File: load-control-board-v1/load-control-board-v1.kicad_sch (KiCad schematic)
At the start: 10 parts, among them Q1 BSC026N08NS5, U1 LM741

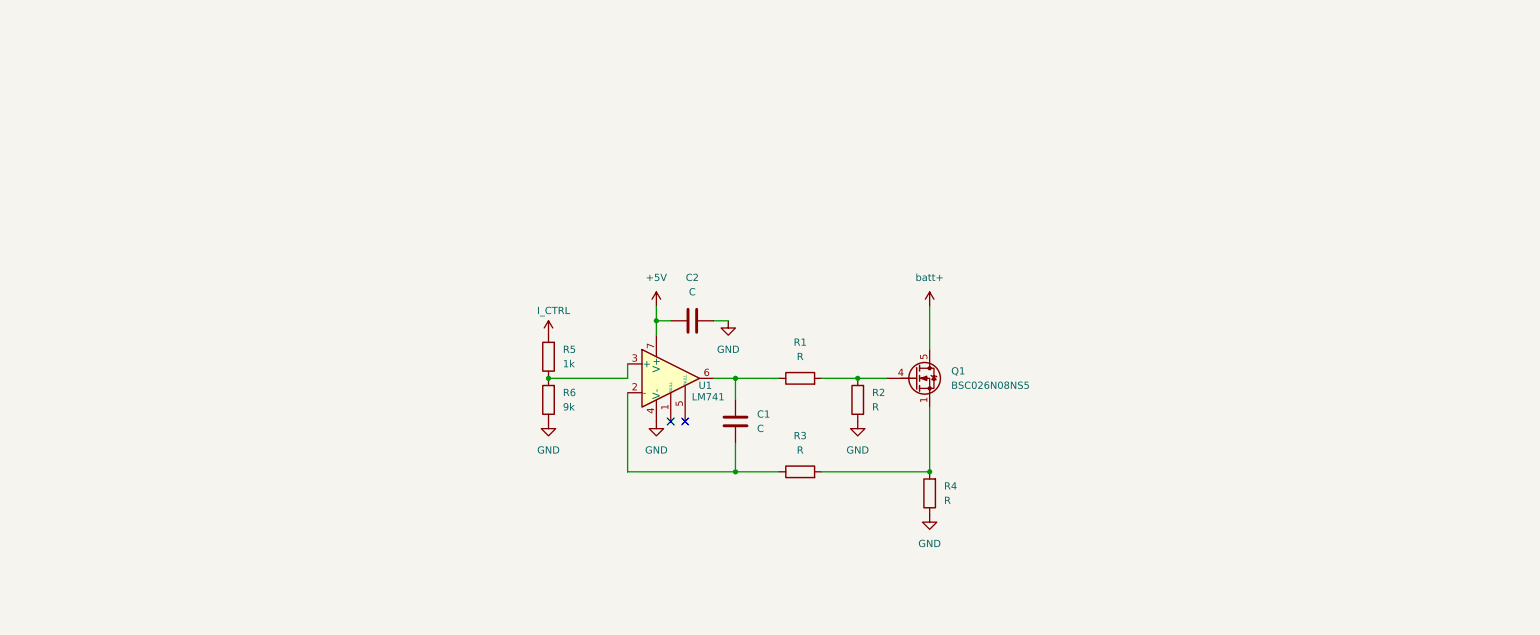
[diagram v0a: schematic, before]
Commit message: communicate 1
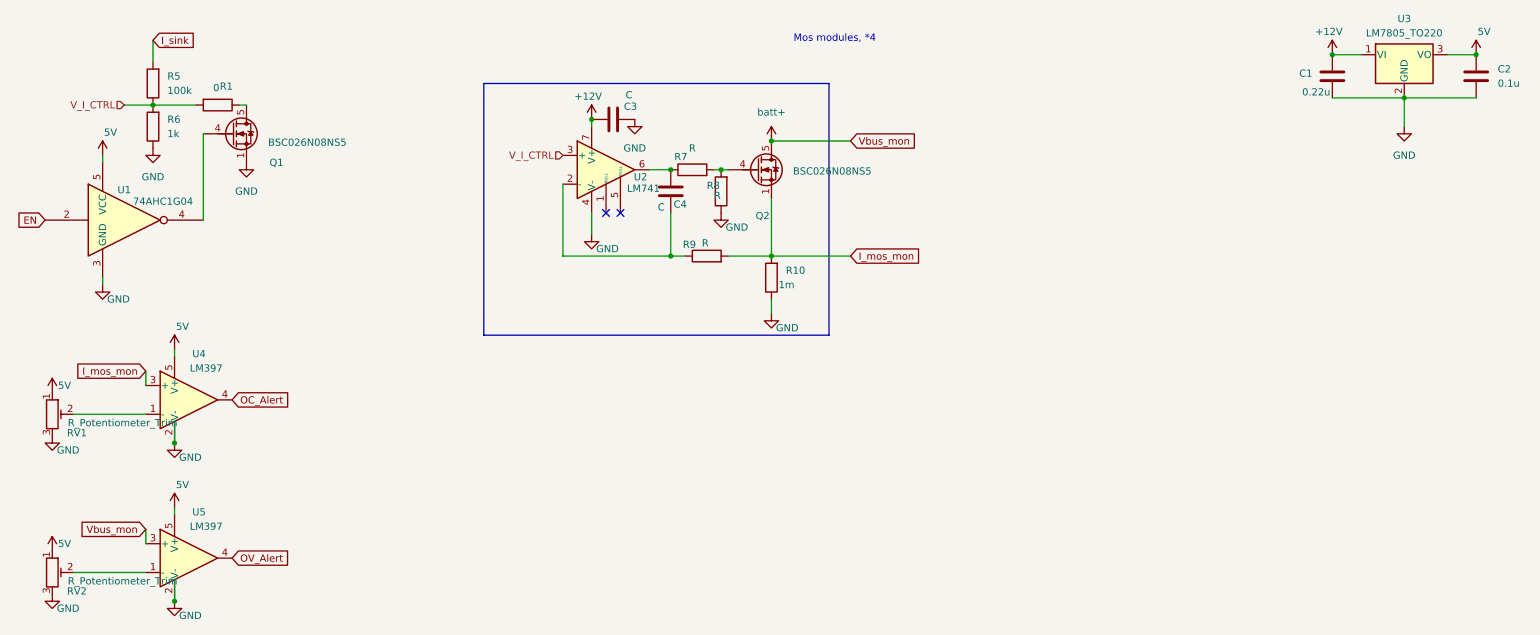
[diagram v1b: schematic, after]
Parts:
- removed R2, R3, R4: R, symbol Device:R
- removed U1: LM741, symbol Amplifier_Operational:LM741
- added C3, C4: C, symbol Device:C
- added Q2: BSC026N08NS5, Package_TO_SOT_SMD:TDSON-8-1, symbol Transistor_FET:BSC026N08NS5
- added R10: 1m, symbol Device:R
- added R7, R8, R9: R, symbol Device:R
- added RV1, RV2: R_Potentiometer_Trim, symbol Device:R_Potentiometer_Trim
- added U1: 74AHC1G04, symbol 74xGxx:74AHC1G04
- added U2: LM741, symbol Amplifier_Operational:LM741
- added U3: LM7805_TO220, Package_TO_SOT_THT:TO-220-3_Vertical, symbol Regulator_Linear:LM7805_TO220
- added U4, U5: LM397, Package_TO_SOT_SMD:SOT-23-5, symbol Comparator:LM397
- C1: value C -> 0.22u
- C2: value C -> 0.1u
- R1: value R -> 0
- R5: value 1k -> 100k
- R6: value 9k -> 1k
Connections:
- net GND: now also C1.2, Q1.1 (S), Q1.2 (S), Q1.3 (S), C3.2, R10.1, R8.1, RV1.3, RV2.3, U1.3 (GND), U2.4 (V-), U3.2 (GND), U4.2 (V-), U5.2 (V-)
- net batt+: now also Q2.5 (D), U5.3 (+); no longer Q1.5 (D)
- net at R1.1: now also Q1.5 (D); no longer C1.1
- net at Q1.4 (G): now also U1.4; no longer R1.2
- net V_I_CTRL: now reaches R5.1, R6.2
- net V_I_CTRL: now also R1.2, U2.3 (+)
- net +5V renamed 5V
- net 5V: now also RV1.1, RV2.1, U1.5 (VCC), U3.3 (VO), U4.5 (V+), U5.5 (V+)
- net I_CTRL renamed I_sink
- new net: RV2.2, U5.1 (-)
- new net: C4.1, R7.1, U2.6
- new net: Q2.4 (G), R7.2, R8.2
- new net: C4.2, R9.1, U2.2 (-)
- new net: RV1.2, U4.1 (-)
- new net +12V: C1.1, C3.1, U2.7 (V+), U3.1 (VI)
- new net EN: U1.2
- new net I_mos_mon: Q2.1 (S), Q2.2 (S), Q2.3 (S), R10.2, R9.2, U4.3 (+)
- new net OC_Alert: U4.4
- new net OV_Alert: U5.4
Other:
- note added: "Mos modules, *4"
- moved on the sheet: R5, R6
